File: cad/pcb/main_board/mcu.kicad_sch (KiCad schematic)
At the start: 10 parts, among them SW1 SW_DIP_x02, U1 STM32F401R_B-C_Tx, Y1 Crystal_GND23

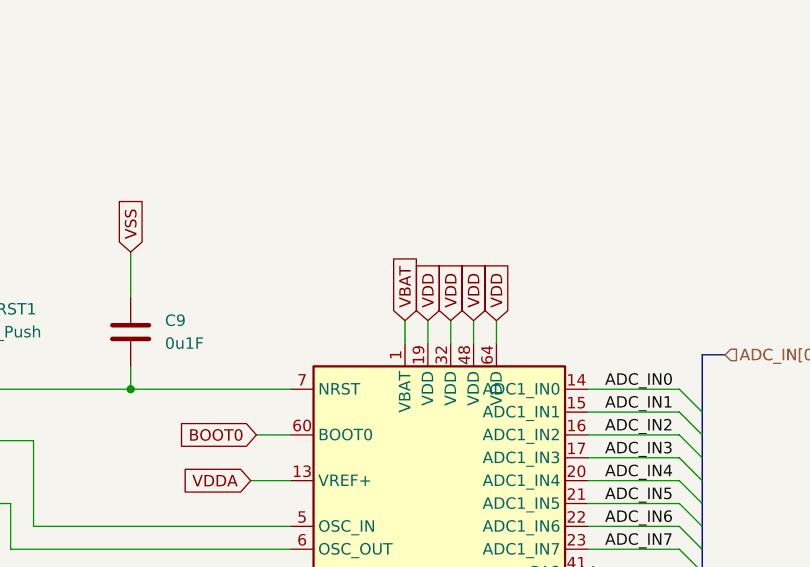
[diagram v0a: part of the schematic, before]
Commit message: Thermo Couple Pins
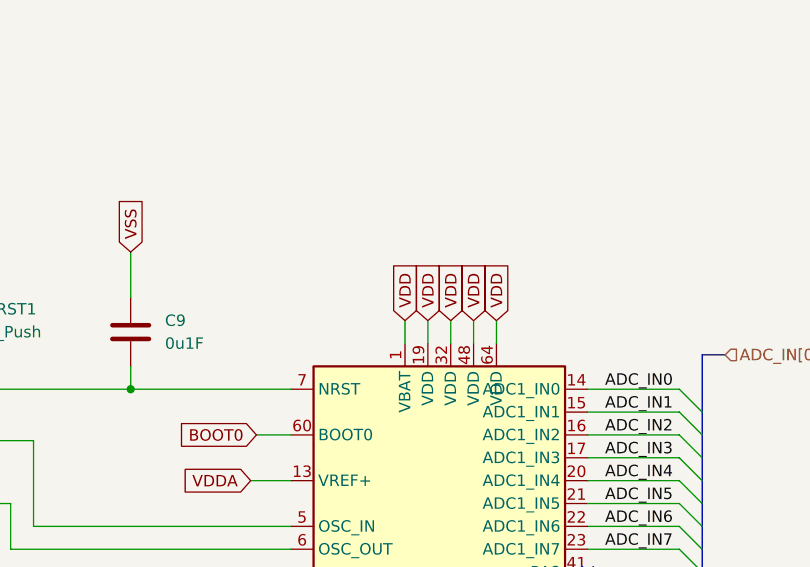
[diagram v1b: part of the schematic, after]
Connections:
- net VBAT is gone; now on net VDD: U1.1 (VBAT)
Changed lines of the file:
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@@
+    )
+  )
+  (global_label "VDD" (shape input) (at 164.465 52.07 90) (fields_autoplaced)
+    (effects (font (size 1.27 1.27)) (justify left))
+    (property "Intersheetrefs" "${INTERSHEET_REFS}" (at 164.465 45.4562 90)
+      (effects (font (size 1.27 1.27)) (justify left) hide)
     )
   )
@@
       (effects (font (size 1.27 1.27)) (justify left) hide)
     )
-  )
-  (global_label "VBAT" (shape input) (at 164.465 52.07 90) (fields_autoplaced)
-    (effects (font (size 1.27 1.27)) (justify left))
-    (property "Intersheetrefs" "${INTERSHEET_REFS}" (at 164.465 44.67 90)
-      (effects (font (size 1.27 1.27)) (justify left) hide)
-    )
